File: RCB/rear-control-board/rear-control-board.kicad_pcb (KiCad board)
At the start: 2 copper layers, 99.7 x 113 mm, 69 parts, among them J1 Conn_01x23, J2 Conn_01x23, J3 Conn_01x08, J4 JST-B2B-VERT-2PIN, J5 JST-B2B-VERT-2PIN, J6 FTSH-107-01-F-DV-K, K1 T9VV1K15-12S, K2 G5V-2, K3 G5V-2, U1 STM32F413CGUx, U3 LDL1117S33R, U4 MAX33054EASA+T, U5 BV1HAL45EFJ, U6 BV1HAL45EFJ, U7 BV1HAL45EFJ, Y1 CSTNE8M00

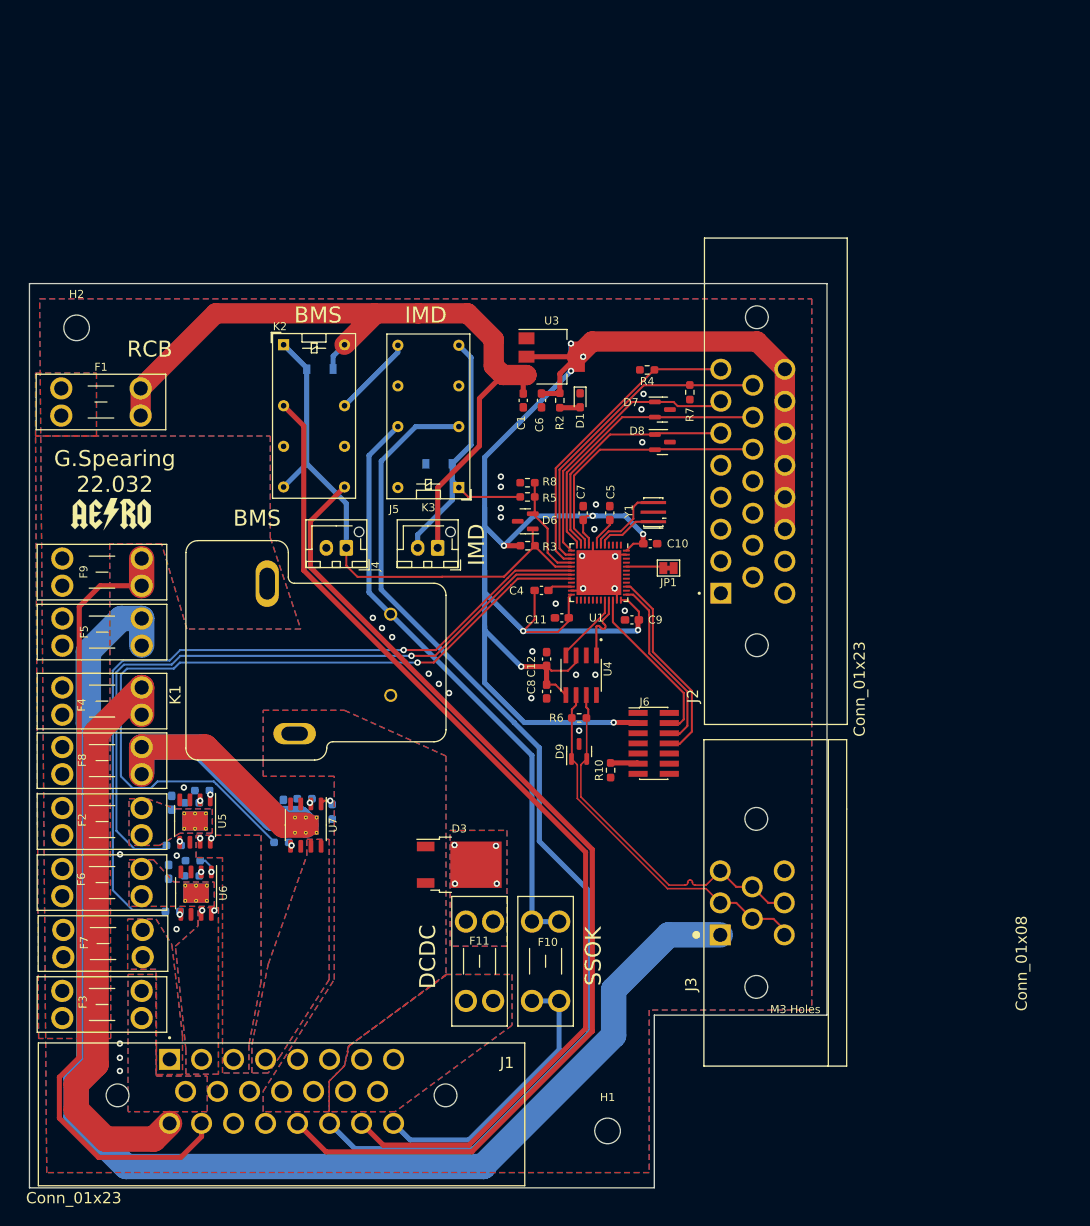
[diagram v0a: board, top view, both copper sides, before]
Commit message: updating layout notes
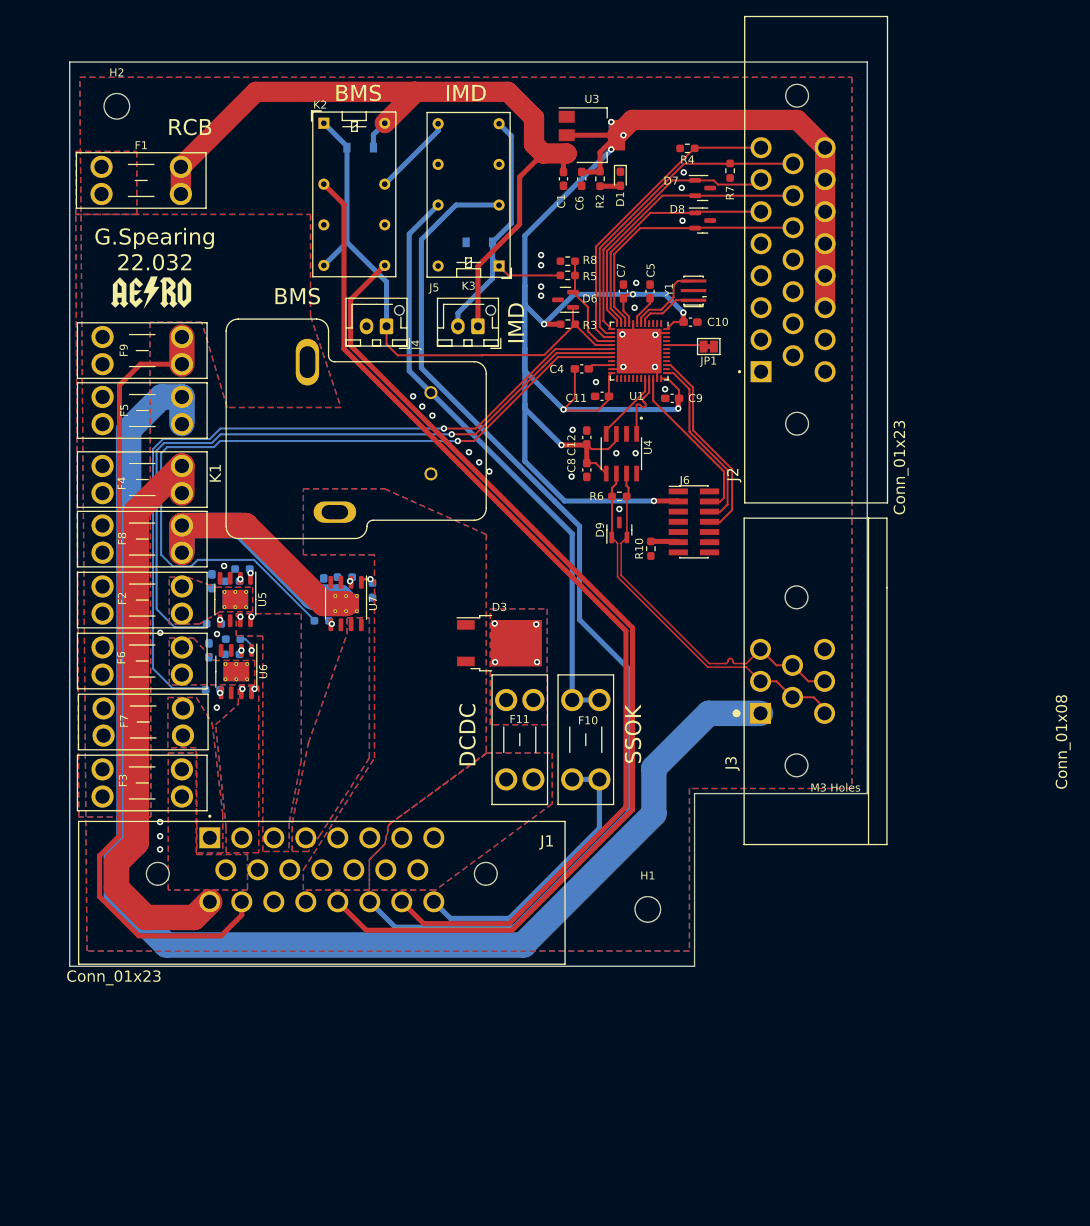
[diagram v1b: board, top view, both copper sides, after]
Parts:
- moved C11 28.1 mm to (145.2, 69.3)
- moved C13 28.1 mm to (110.4, 93.0)
- moved H1 28.1 mm to (151.0, 133.5)
- moved J2 28.1 mm to (165.1, 66.3)
- moved K1 28.1 mm to (111.8, 74.4)
- moved U7 28.1 mm to (113.2, 95.2)
- moved C10 28.1 mm to (156.3, 60.1)
- moved D8 28.1 mm to (157.8, 47.4)
- moved JP1 28.1 mm to (158.6, 63.1)
- moved K2 28.1 mm to (110.5, 35.2)
- moved R4 28.1 mm to (155.9, 38.3)
- moved R5 28.1 mm to (140.9, 54.2)
- moved R7 28.1 mm to (161.2, 41.1)
- moved C1 28.1 mm to (140.4, 42.2)
- moved C12 28.1 mm to (143.3, 74.5)
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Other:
- board text removed: "bring decaps closer can pins on connect doens't need to be big use stm32 standard programming header, 5x10 1.27 pitch -> harwin (the one on the stlink mini) from stm32 go 2.54 then larger (15mil) add via near decoupling pins on caps use 8mil trace minimum check zone spacing, min is 8/8 (thickness/spacing) higher for 12V"

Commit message: touching up layout and making gerbers
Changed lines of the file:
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@@
       (outputformat 1)
       (mirror false)
-      (drillshape 1)
+      (drillshape 0)
       (scaleselection 1)
-      (outputdirectory "")
+      (outputdirectory "RCB_Gerber/")
     )
   )
@@
     (fp_line (start 0 -1.35) (end 0.625 -2.35) (layer "F.Fab") (width 0.1))
     (pad "" np_thru_hole circle locked (at -1.6 2 180) (size 1.2 1.2) (drill 1.2) (layers *.Cu *.Mask))
-    (pad "1" thru_hole roundrect locked (at 0 0 180) (size 1.7 2) (drill 1) (layers *.Cu *.Mask) (roundrect_rratio 0.147059)
+    (pad "1" thru_hole roundrect locked (at 0 0 180) (size 1.7 2) (drill 1) (layers *.Cu *.Mask) (roundrect_rratio 0.1470588235)
       (net 8 "/FAULT_LATCHER/BMS_SWITCH") (pinfunction "Pin_1") (pintype "passive"))
     (pad "2" thru_hole oval locked (at 2.5 0 180) (size 1.7 2) (drill 1) (layers *.Cu *.Mask)
@@
     (fp_line (start 3.5 -3.5) (end 3.5 3.5) (layer "F.Fab") (width 0.1))
     (fp_line (start 3.5 3.5) (end -3.5 3.5) (layer "F.Fab") (width 0.1))
-    (pad "" smd roundrect locked (at -2.1 0.7 270) (size 1.13 1.13) (layers "F.Paste") (roundrect_rratio 0.221239))
-    (pad "" smd roundrect locked (at -0.7 2.1 270) (size 1.13 1.13) (layers "F.Paste") (roundrect_rratio 0.221239))
-    (pad "" smd roundrect locked (at -0.7 -0.7 270) (size 1.13 1.13) (layers "F.Paste") (roundrect_rratio 0.221239))
-    (pad "" smd roundrect locked (at 0.7 2.1 270) (size 1.13 1.13) (layers "F.Paste") (roundrect_rratio 0.221239))
-    (pad "" smd roundrect locked (at 0.7 -0.7 270) (size 1.13 1.13) (layers "F.Paste") (roundrect_rratio 0.221239))
-    (pad "" smd roundrect locked (at -2.1 -2.1 270) (size 1.13 1.13) (layers "F.Paste") (roundrect_rratio 0.221239))
-    (pad "" smd roundrect locked (at 2.1 -0.7 270) (size 1.13 1.13) (layers "F.Paste") (roundrect_rratio 0.221239))
-    (pad "" smd roundrect locked (at 2.1 2.1 270) (size 1.13 1.13) (layers "F.Paste") (roundrect_rratio 0.221239))
-    (pad "" smd roundrect locked (at 0.7 -2.1 270) (size 1.13 1.13) (layers "F.Paste") (roundrect_rratio 0.221239))
-    (pad "" smd roundrect locked (at 0.7 0.7 270) (size 1.13 1.13) (layers "F.Paste") (roundrect_rratio 0.221239))
-    (pad "" smd roundrect locked (at -0.7 0.7 270) (size 1.13 1.13) (layers "F.Paste") (roundrect_rratio 0.221239))
-    (pad "" smd roundrect locked (at 2.1 0.7 270) (size 1.13 1.13) (layers "F.Paste") (roundrect_rratio 0.221239))
-    (pad "" smd roundrect locked (at -0.7 -2.1 270) (size 1.13 1.13) (layers "F.Paste") (roundrect_rratio 0.221239))
-    (pad "" smd roundrect locked (at 2.1 -2.1 270) (size 1.13 1.13) (layers "F.Paste") (roundrect_rratio 0.221239))
-    (pad "" smd roundrect locked (at -2.1 2.1 270) (size 1.13 1.13) (layers "F.Paste") (roundrect_rratio 0.221239))
-    (pad "" smd roundrect locked (at -2.1 -0.7 270) (size 1.13 1.13) (layers "F.Paste") (roundrect_rratio 0.221239))
+    (pad "" smd roundrect locked (at -2.1 0.7 270) (size 1.13 1.13) (layers "F.Paste") (roundrect_rratio 0.2212389381))
+    (pad "" smd roundrect locked (at -0.7 2.1 270) (size 1.13 1.13) (layers "F.Paste") (roundrect_rratio 0.2212389381))
+    (pad "" smd roundrect locked (at -0.7 -0.7 270) (size 1.13 1.13) (layers "F.Paste") (roundrect_rratio 0.2212389381))
+    (pad "" smd roundrect locked (at 0.7 2.1 270) (size 1.13 1.13) (layers "F.Paste") (roundrect_rratio 0.2212389381))
+    (pad "" smd roundrect locked (at 0.7 -0.7 270) (size 1.13 1.13) (layers "F.Paste") (roundrect_rratio 0.2212389381))
+    (pad "" smd roundrect locked (at -2.1 -2.1 270) (size 1.13 1.13) (layers "F.Paste") (roundrect_rratio 0.2212389381))
+    (pad "" smd roundrect locked (at 2.1 -0.7 270) (size 1.13 1.13) (layers "F.Paste") (roundrect_rratio 0.2212389381))
+    (pad "" smd roundrect locked (at 2.1 2.1 270) (size 1.13 1.13) (layers "F.Paste") (roundrect_rratio 0.2212389381))
+    (pad "" smd roundrect locked (at 0.7 -2.1 270) (size 1.13 1.13) (layers "F.Paste") (roundrect_rratio 0.2212389381))
+    (pad "" smd roundrect locked (at 0.7 0.7 270) (size 1.13 1.13) (layers "F.Paste") (roundrect_rratio 0.2212389381))
+    (pad "" smd roundrect locked (at -0.7 0.7 270) (size 1.13 1.13) (layers "F.Paste") (roundrect_rratio 0.2212389381))
+    (pad "" smd roundrect locked (at 2.1 0.7 270) (size 1.13 1.13) (layers "F.Paste") (roundrect_rratio 0.2212389381))
+    (pad "" smd roundrect locked (at -0.7 -2.1 270) (size 1.13 1.13) (layers "F.Paste") (roundrect_rratio 0.2212389381))
+    (pad "" smd roundrect locked (at 2.1 -2.1 270) (size 1.13 1.13) (layers "F.Paste") (roundrect_rratio 0.2212389381))
+    (pad "" smd roundrect locked (at -2.1 2.1 270) (size 1.13 1.13) (layers "F.Paste") (roundrect_rratio 0.2212389381))
+    (pad "" smd roundrect locked (at -2.1 -0.7 270) (size 1.13 1.13) (layers "F.Paste") (roundrect_rratio 0.2212389381))
     (pad "1" smd roundrect locked (at -3.4375 -2.75 270) (size 0.875 0.25) (layers "F.Cu" "F.Paste" "F.Mask") (roundrect_rratio 0.25)
       (net 61 "unconnected-(U1-Pad1)") (pinfunction "VBAT") (pintype "power_in"))
@@
     (fp_line (start -2.45 3.4) (end 4.95 3.4) (layer "F.Fab") (width 0.1))
     (pad "" np_thru_hole circle locked (at -1.6 2 180) (size 1.2 1.2) (drill 1.2) (layers *.Cu *.Mask))
-    (pad "1" thru_hole roundrect locked (at 0 0 180) (size 1.7 2) (drill 1) (layers *.Cu *.Mask) (roundrect_rratio 0.147059)
+    (pad "1" thru_hole roundrect locked (at 0 0 180) (size 1.7 2) (drill 1) (layers *.Cu *.Mask) (roundrect_rratio 0.1470588235)
       (net 3 "INT_12V") (pinfunction "Pin_1") (pintype "passive"))
     (pad "2" thru_hole oval locked (at 2.5 0 180) (size 1.7 2) (drill 1) (layers *.Cu *.Mask)
